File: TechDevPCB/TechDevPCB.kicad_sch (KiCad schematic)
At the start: 51 parts, among them J1 Screw_Terminal_01x02, J10 Conn_01x05_Pin, J11 Conn_01x01_Socket, J12 Screw_Terminal_01x04, J13 Conn_01x01_Socket, J14 Conn_01x01_Socket, J15 Conn_01x01_Socket, J16 Conn_01x01_Socket, J17 Conn_01x01_Socket, J18 Conn_01x01_Socket, J19 Conn_01x01_Socket, J2 Screw_Terminal_01x02, J20 Conn_01x01_Socket, J21 Conn_01x01_Socket, J22 Conn_01x01_Socket, J23 Conn_01x01_Socket, J24 Conn_01x01_Socket, J25 Conn_01x01_Socket, J26 Conn_01x01_Socket, J27 Conn_01x01_Socket, J28 Conn_01x01_Socket, J29 Conn_01x01_Socket, J3 Conn_01x02_Pin, J30 Conn_01x01_Socket, J31 Conn_01x01_Socket, J4 Screw_Terminal_01x04, J5 Conn_01x02_Pin, J6 Conn_01x05_Pin, J7 Conn_01x04_Pin, J8 Conn_01x05_Pin, J9 Conn_01x05_Pin, U1 DRV8825_STEPPER_MOTOR_DRIVER_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, U2 DRV8825_STEPPER_MOTOR_DRIVER_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, U3 XL6009 Boost Converter

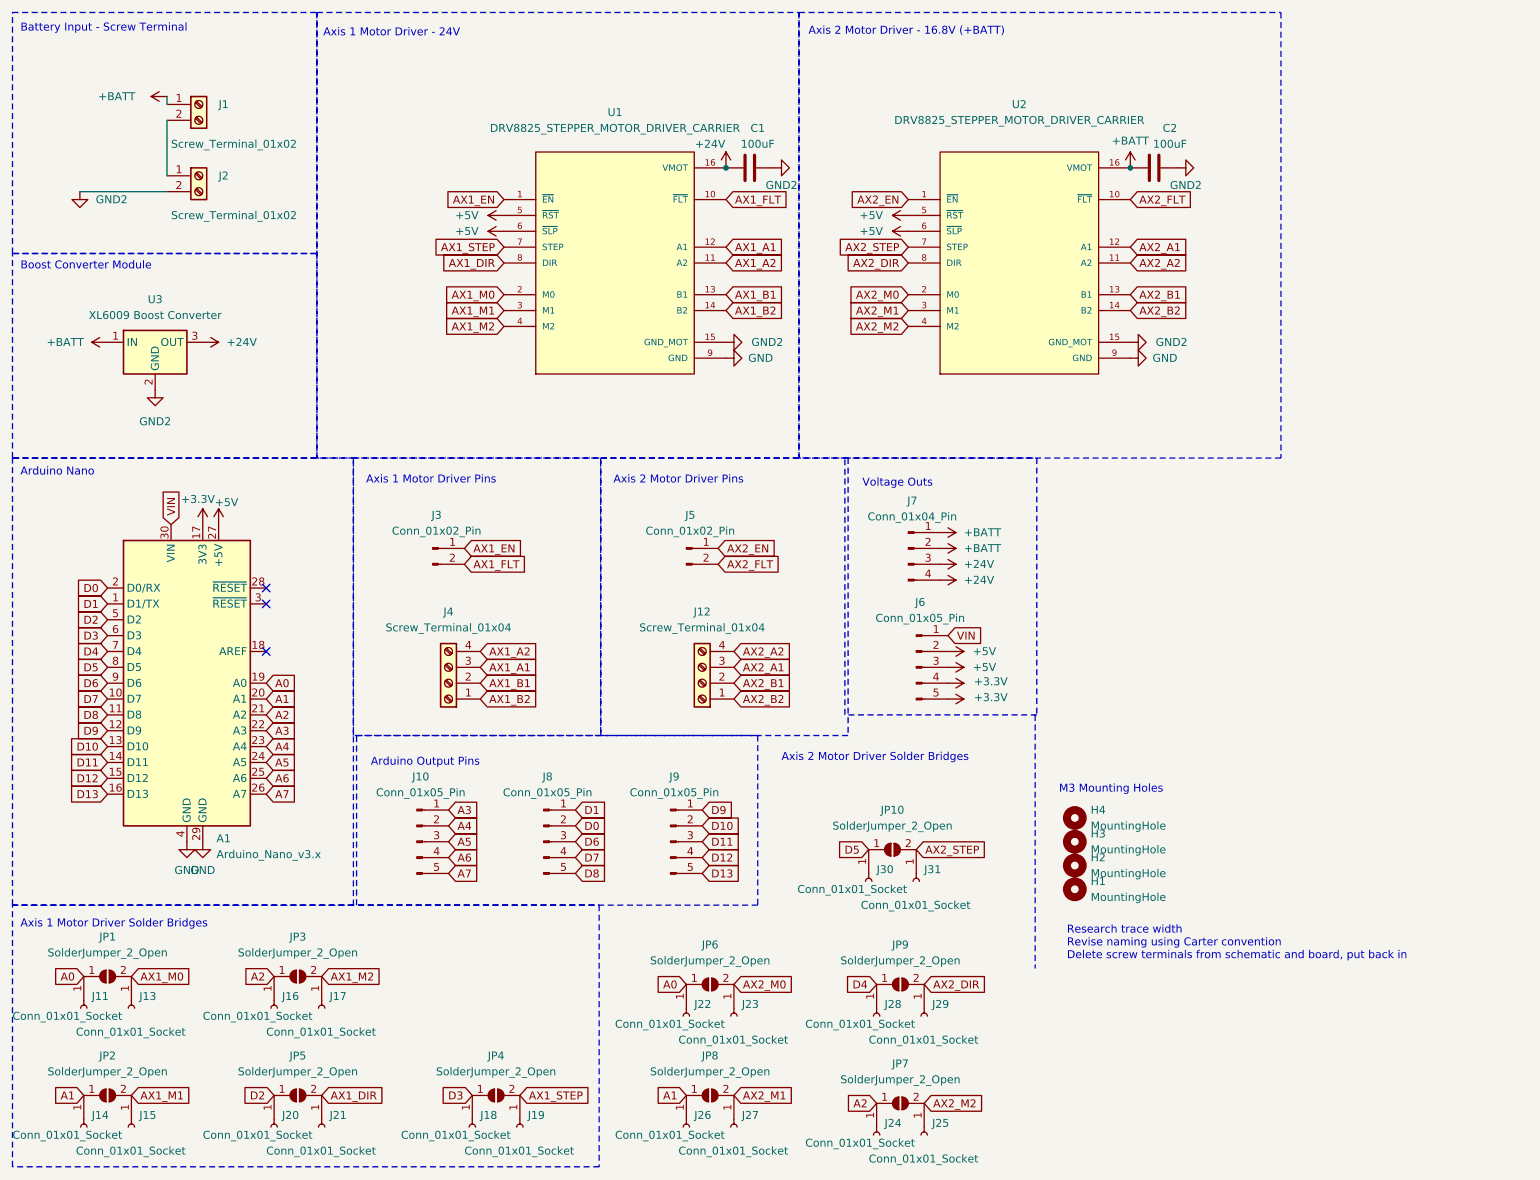
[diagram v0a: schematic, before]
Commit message: PCB Updates
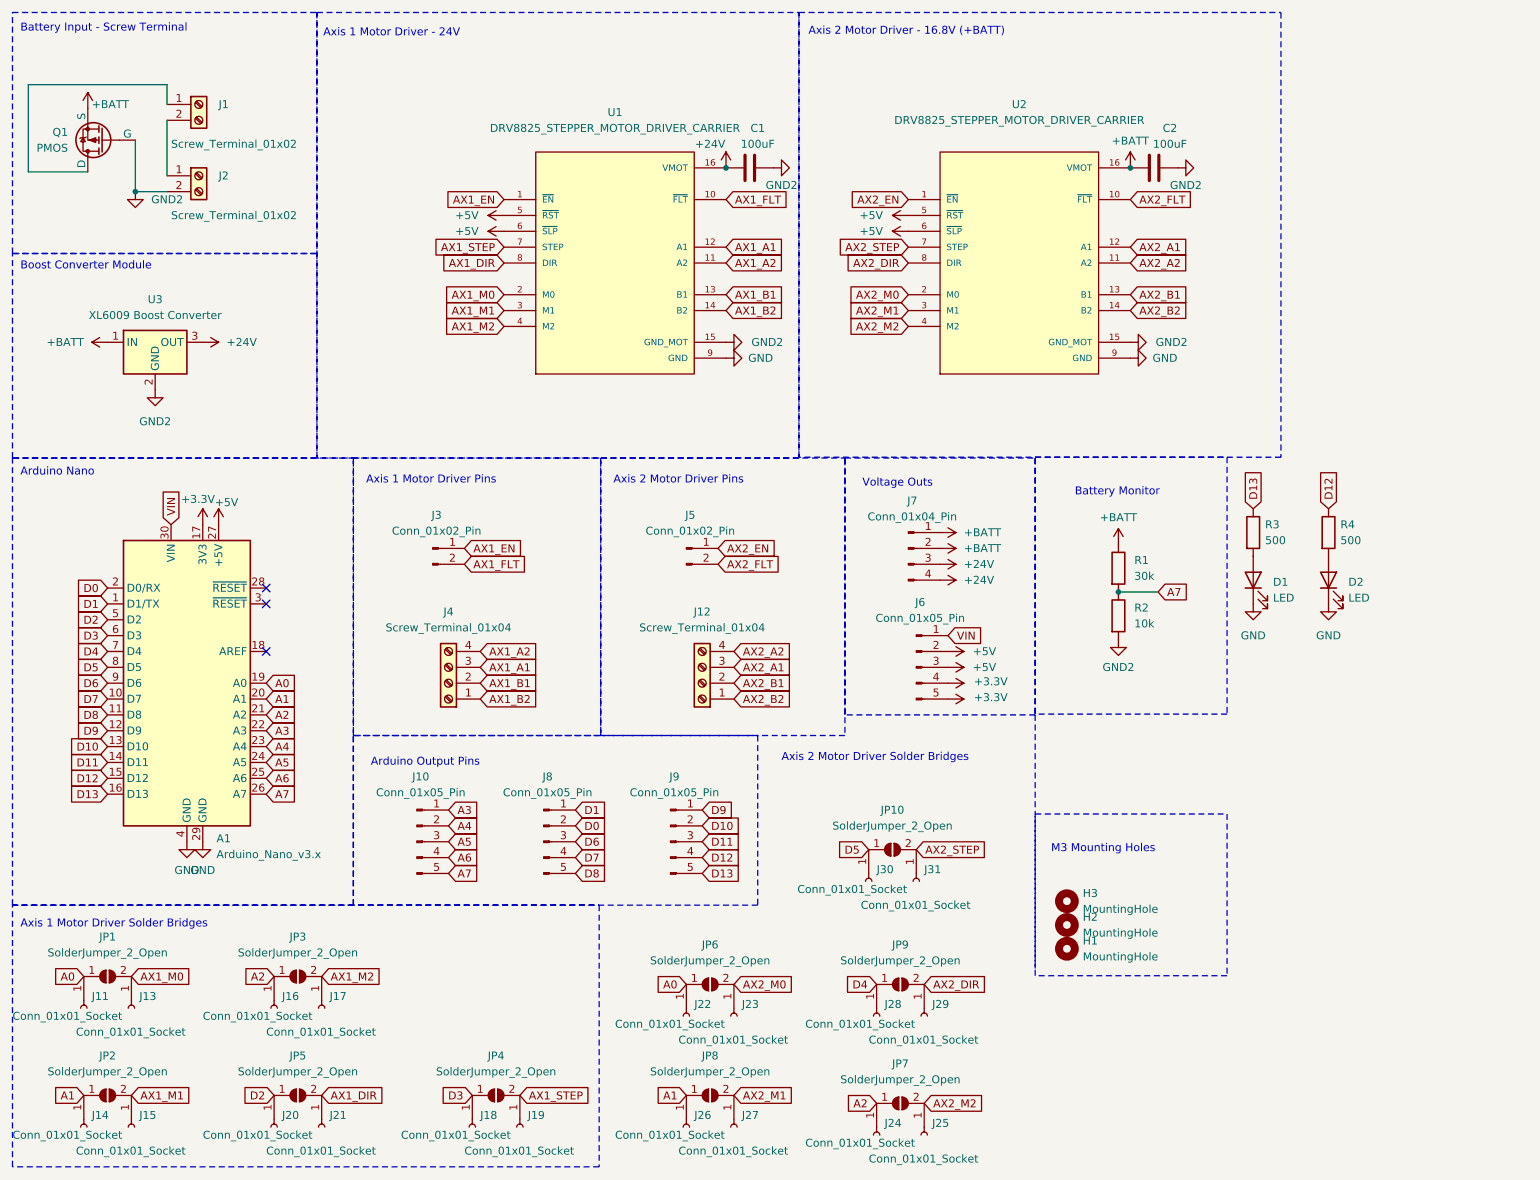
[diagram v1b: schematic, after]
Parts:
- removed H4: MountingHole, MountingHole:MountingHole_3.2mm_M3_DIN965, symbol Mechanical:MountingHole
- added D1, D2: LED, LED_THT:LED_Rectangular_W3.0mm_H2.0mm, symbol Device:LED
- added Q1: PMOS, Package_TO_SOT_THT:TO-251-3-1EP_Horizontal_TabDown, symbol Simulation_SPICE:PMOS
- added R1: 30k, Resistor_THT:R_Axial_DIN0207_L6.3mm_D2.5mm_P10.16mm_Horizontal, symbol Device:R
- added R2: 10k, Resistor_THT:R_Axial_DIN0207_L6.3mm_D2.5mm_P10.16mm_Horizontal, symbol Device:R
- added R3, R4: 500, Resistor_THT:R_Axial_DIN0207_L6.3mm_D2.5mm_P10.16mm_Horizontal, symbol Device:R
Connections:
- net +BATT: now also Q1.3 (S), R1.1; no longer J1.1 (Pin_1)
- net A7: now also R1.2, R2.1
- net D12: now also R4.1
- net D13: now also R3.1
- net GND: now also D1.1 (K), D2.1 (K)
- net GND2: now also Q1.2 (G), R2.2
- new net: D1.2 (A), R3.2
- new net: D2.2 (A), R4.2
- new net: J1.1 (Pin_1), Q1.1 (D)
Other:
- note added: "Battery Monitor"
- note removed: "Research trace width Revise naming using Carter convention Delete screw terminals from schematic and board, put back in"
- moved on the sheet: H1, H2, H3

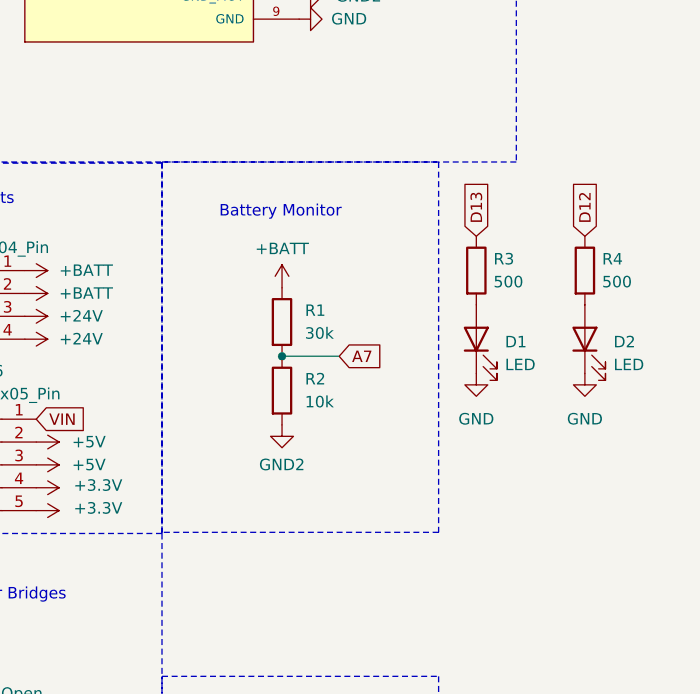
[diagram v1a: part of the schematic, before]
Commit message: PCB Updates
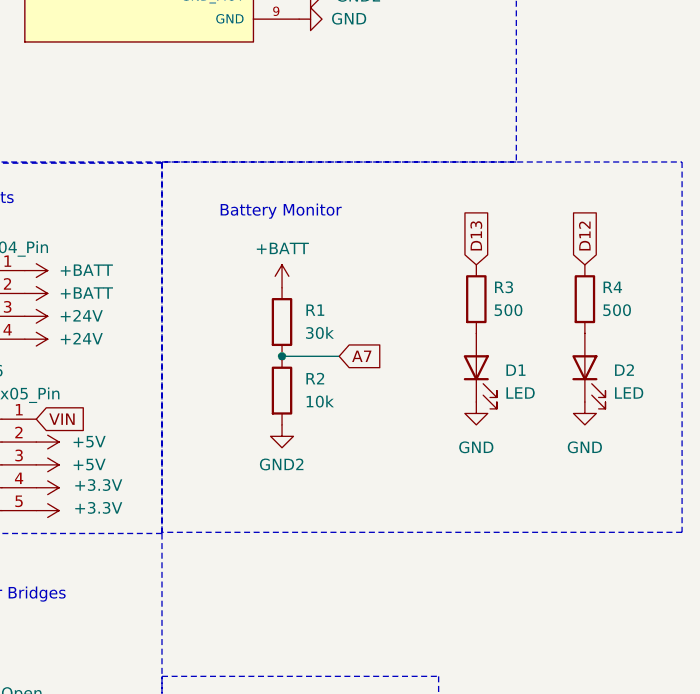
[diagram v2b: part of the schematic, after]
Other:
- moved on the sheet: D1, D2, R3, R4
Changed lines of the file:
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@@
     (fill (type none))
   )
-  (rectangle (start 176.53 83.185) (end 207.264 124.333)
+  (rectangle (start 176.53 83.185) (end 234.315 124.333)
     (stroke (width 0) (type dash))
     (fill (type none))
@@
     )
   )
-  (global_label "D13" (shape input) (at 211.455 91.44 90) (fields_autoplaced)
-    (effects (font (size 1.27 1.27)) (justify left))
-    (property "Intersheetrefs" "${INTERSHEET_REFS}" (at 211.455 84.7658 90)
+  (global_label "D13" (shape input) (at 211.455 94.615 90) (fields_autoplaced)
+    (effects (font (size 1.27 1.27)) (justify left))
+    (property "Intersheetrefs" "${INTERSHEET_REFS}" (at 211.455 87.9408 90)
       (effects (font (size 1.27 1.27)) (justify left) hide)
     )
@@
     )
   )
-  (global_label "D12" (shape input) (at 223.52 91.44 90) (fields_autoplaced)
-    (effects (font (size 1.27 1.27)) (justify left))
-    (property "Intersheetrefs" "${INTERSHEET_REFS}" (at 223.52 84.7658 90)
+  (global_label "D12" (shape input) (at 223.52 94.615 90) (fields_autoplaced)
+    (effects (font (size 1.27 1.27)) (justify left))
+    (property "Intersheetrefs" "${INTERSHEET_REFS}" (at 223.52 87.9408 90)
       (effects (font (size 1.27 1.27)) (justify left) hide)
     )
@@
     )
   )
-  (symbol (lib_id "Device:R") (at 211.455 95.25 0) (unit 1)
-    (in_bom yes) (on_board yes) (dnp no) (fields_autoplaced)
-    (property "Reference" "R3" (at 213.36 93.98 0)
-      (effects (font (size 1.27 1.27)) (justify left))
-    )
-    (property "Value" "500" (at 213.36 96.52 0)
-      (effects (font (size 1.27 1.27)) (justify left))
-    )
-    (property "Footprint" "Resistor_THT:R_Axial_DIN0207_L6.3mm_D2.5mm_P10.16mm_Horizontal" (at 209.677 95.25 90)
-      (effects (font (size 1.27 1.27)) hide)
-    )
-    (property "Datasheet" "~" (at 211.455 95.25 0)
+  (symbol (lib_id "Device:R") (at 211.455 98.425 0) (unit 1)
+    (in_bom yes) (on_board yes) (dnp no) (fields_autoplaced)
+    (property "Reference" "R3" (at 213.36 97.155 0)
+      (effects (font (size 1.27 1.27)) (justify left))
+    )
+    (property "Value" "500" (at 213.36 99.695 0)
+      (effects (font (size 1.27 1.27)) (justify left))
+    )
+    (property "Footprint" "Resistor_THT:R_Axial_DIN0207_L6.3mm_D2.5mm_P10.16mm_Horizontal" (at 209.677 98.425 90)
+      (effects (font (size 1.27 1.27)) hide)
+    )
+    (property "Datasheet" "~" (at 211.455 98.425 0)
       (effects (font (size 1.27 1.27)) hide)
     )
@@
     )
   )
-  (symbol (lib_id "Device:R") (at 223.52 95.25 0) (unit 1)
-    (in_bom yes) (on_board yes) (dnp no) (fields_autoplaced)
-    (property "Reference" "R4" (at 225.425 93.98 0)
-      (effects (font (size 1.27 1.27)) (justify left))
-    )
-    (property "Value" "500" (at 225.425 96.52 0)
-      (effects (font (size 1.27 1.27)) (justify left))
-    )
-    (property "Footprint" "Resistor_THT:R_Axial_DIN0207_L6.3mm_D2.5mm_P10.16mm_Horizontal" (at 221.742 95.25 90)
-      (effects (font (size 1.27 1.27)) hide)
-    )
-    (property "Datasheet" "~" (at 223.52 95.25 0)
+  (symbol (lib_id "Device:R") (at 223.52 98.425 0) (unit 1)
+    (in_bom yes) (on_board yes) (dnp no) (fields_autoplaced)
+    (property "Reference" "R4" (at 225.425 97.155 0)
+      (effects (font (size 1.27 1.27)) (justify left))
+    )
+    (property "Value" "500" (at 225.425 99.695 0)
+      (effects (font (size 1.27 1.27)) (justify left))
+    )
+    (property "Footprint" "Resistor_THT:R_Axial_DIN0207_L6.3mm_D2.5mm_P10.16mm_Horizontal" (at 221.742 98.425 90)
+      (effects (font (size 1.27 1.27)) hide)
+    )
+    (property "Datasheet" "~" (at 223.52 98.425 0)
       (effects (font (size 1.27 1.27)) hide)
     )
@@
     )
   )
-  (symbol (lib_id "Device:LED") (at 223.52 102.87 90) (unit 1)
-    (in_bom yes) (on_board yes) (dnp no) (fields_autoplaced)
-    (property "Reference" "D2" (at 226.695 103.1875 90)
+  (symbol (lib_id "Device:LED") (at 223.52 106.045 90) (unit 1)
+    (in_bom yes) (on_board yes) (dnp no) (fields_autoplaced)
+    (property "Reference" "D2" (at 226.695 106.3625 90)
       (effects (font (size 1.27 1.27)) (justify right))
     )
-    (property "Value" "LED" (at 226.695 105.7275 90)
+    (property "Value" "LED" (at 226.695 108.9025 90)
       (effects (font (size 1.27 1.27)) (justify right))
     )
-    (property "Footprint" "LED_THT:LED_Rectangular_W3.0mm_H2.0mm" (at 223.52 102.87 0)
-      (effects (font (size 1.27 1.27)) hide)
-    )
-    (property "Datasheet" "~" (at 223.52 102.87 0)
+    (property "Footprint" "LED_THT:LED_Rectangular_W3.0mm_H2.0mm" (at 223.52 106.045 0)
+      (effects (font (size 1.27 1.27)) hide)
+    )
+    (property "Datasheet" "~" (at 223.52 106.045 0)
       (effects (font (size 1.27 1.27)) hide)
     )
@@
     )
   )
-  (symbol (lib_id "power:GND") (at 223.52 106.68 0) (unit 1)
-    (in_bom yes) (on_board yes) (dnp no) (fields_autoplaced)
-    (property "Reference" "#PWR033" (at 223.52 113.03 0)
-      (effects (font (size 1.27 1.27)) hide)
-    )
-    (property "Value" "GND" (at 223.52 111.76 0)
-      (effects (font (size 1.27 1.27)))
-    )
-    (property "Footprint" "" (at 223.52 106.68 0)
-      (effects (font (size 1.27 1.27)) hide)
-    )
-    (property "Datasheet" "" (at 223.52 106.68 0)
+  (symbol (lib_id "power:GND") (at 223.52 109.855 0) (unit 1)
+    (in_bom yes) (on_board yes) (dnp no) (fields_autoplaced)
+    (property "Reference" "#PWR033" (at 223.52 116.205 0)
+      (effects (font (size 1.27 1.27)) hide)
+    )
+    (property "Value" "GND" (at 223.52 114.935 0)
+      (effects (font (size 1.27 1.27)))
+    )
+    (property "Footprint" "" (at 223.52 109.855 0)
+      (effects (font (size 1.27 1.27)) hide)
+    )
+    (property "Datasheet" "" (at 223.52 109.855 0)
       (effects (font (size 1.27 1.27)) hide)
     )
@@
     )
   )
-  (symbol (lib_id "power:GND") (at 211.455 106.68 0) (unit 1)
-    (in_bom yes) (on_board yes) (dnp no) (fields_autoplaced)
-    (property "Reference" "#PWR032" (at 211.455 113.03 0)
-      (effects (font (size 1.27 1.27)) hide)
-    )
-    (property "Value" "GND" (at 211.455 111.76 0)
-      (effects (font (size 1.27 1.27)))
-    )
-    (property "Footprint" "" (at 211.455 106.68 0)
-      (effects (font (size 1.27 1.27)) hide)
-    )
-    (property "Datasheet" "" (at 211.455 106.68 0)
+  (symbol (lib_id "power:GND") (at 211.455 109.855 0) (unit 1)
+    (in_bom yes) (on_board yes) (dnp no) (fields_autoplaced)
+    (property "Reference" "#PWR032" (at 211.455 116.205 0)
+      (effects (font (size 1.27 1.27)) hide)
+    )
+    (property "Value" "GND" (at 211.455 114.935 0)
+      (effects (font (size 1.27 1.27)))
+    )
+    (property "Footprint" "" (at 211.455 109.855 0)
+      (effects (font (size 1.27 1.27)) hide)
+    )
+    (property "Datasheet" "" (at 211.455 109.855 0)
       (effects (font (size 1.27 1.27)) hide)
     )
@@
     )
   )
-  (symbol (lib_id "Device:LED") (at 211.455 102.87 90) (unit 1)
-    (in_bom yes) (on_board yes) (dnp no) (fields_autoplaced)
-    (property "Reference" "D1" (at 214.63 103.1875 90)
+  (symbol (lib_id "Device:LED") (at 211.455 106.045 90) (unit 1)
+    (in_bom yes) (on_board yes) (dnp no) (fields_autoplaced)
+    (property "Reference" "D1" (at 214.63 106.3625 90)
       (effects (font (size 1.27 1.27)) (justify right))
     )
-    (property "Value" "LED" (at 214.63 105.7275 90)
+    (property "Value" "LED" (at 214.63 108.9025 90)
       (effects (font (size 1.27 1.27)) (justify right))
     )
-    (property "Footprint" "LED_THT:LED_Rectangular_W3.0mm_H2.0mm" (at 211.455 102.87 0)
-      (effects (font (size 1.27 1.27)) hide)
-    )
-    (property "Datasheet" "~" (at 211.455 102.87 0)
-      (effects (font (size 1.27 1.27)) hide)
-    )
+    (property "Footprint" "LED_THT:LED_Rectangular_W3.0mm_H2.0mm" (at 211.455 106.045 0)
+      (effects (font (size 1.27 1.27)) hide)
+    )
+    (property "Datasheet" "~" (at 211.455 106.045 0)
+      (effects (font (size 1.27 1.27)) hide)
+    )
